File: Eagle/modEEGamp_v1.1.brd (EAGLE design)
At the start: 100 x 80 mm, 115 parts, among them IC201 TLC277P, IC202 INA114P, IC203 INA114P, IC204 TLC277P, IC205 TLC277P, IC206 TLC277P, J201 PINHD-2X17, P201 20k, P202 20k, P203 20k, Q201 BC557, Q202 BC557, Q203 BC557, Q204 BC557, Q205 BC547, Q206 BC547, Q207 BC547, Q208 BC547

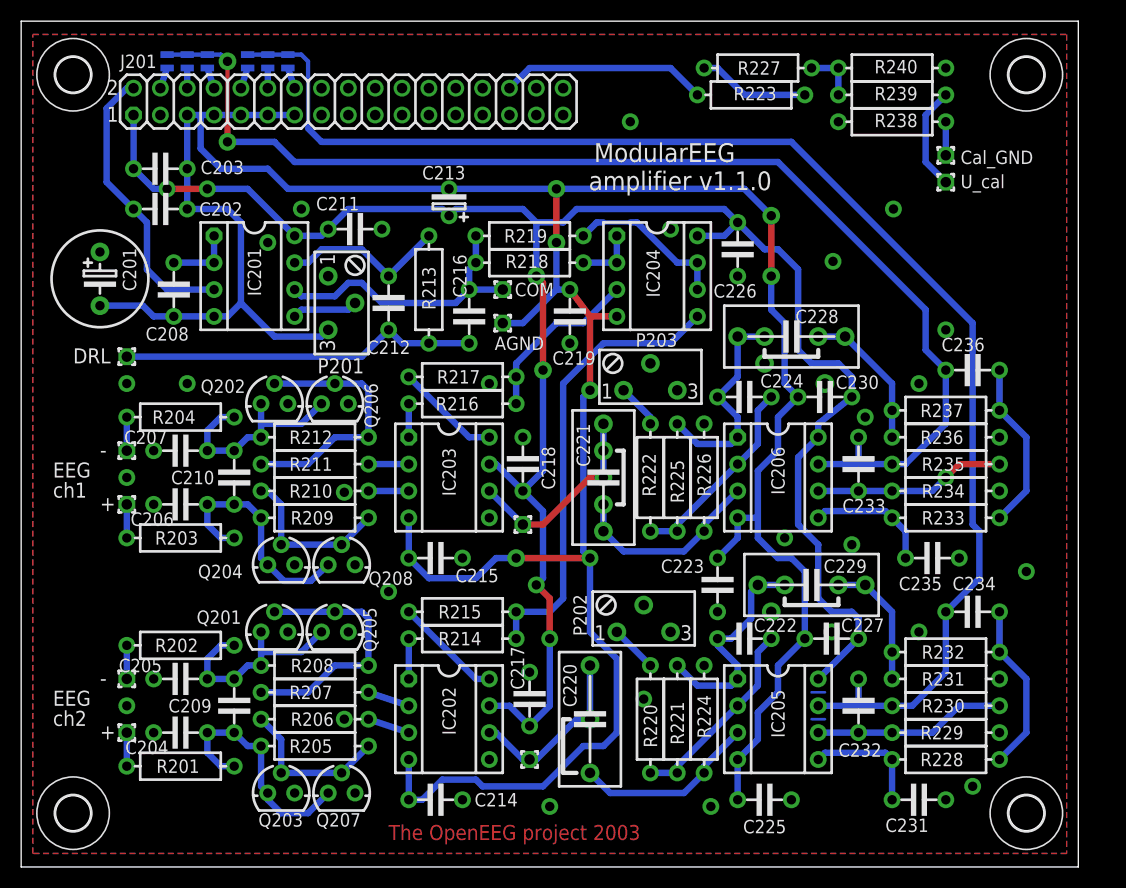
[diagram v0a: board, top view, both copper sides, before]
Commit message: New version!
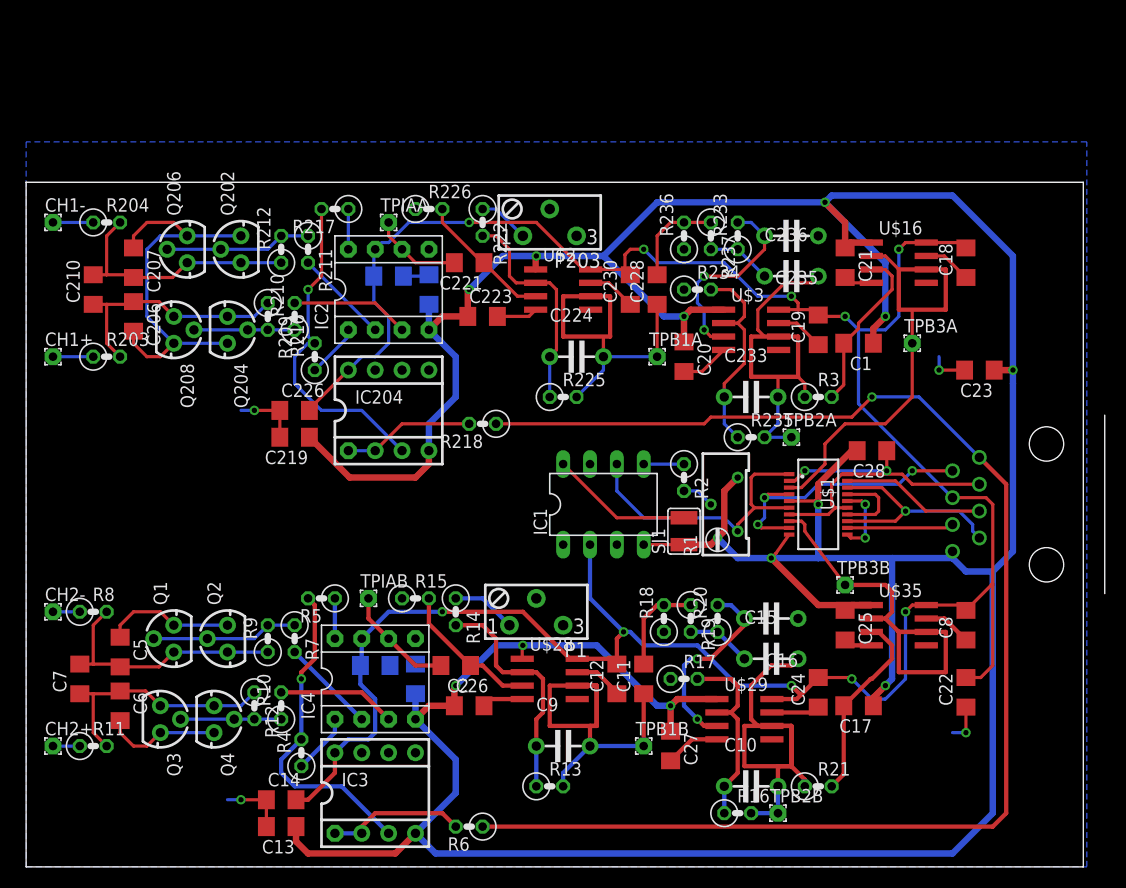
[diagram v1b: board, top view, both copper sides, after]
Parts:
- removed C201: 47µF tan 1ohm, MODEEG:ES-5
- removed C202, C203: 10nF, MODEEG:C-5
- removed C204, C205: 100pF, MODEEG:C-5
- removed C208, C211, C214, C217, C225, C227: 100nF, MODEEG:C-5
- removed C209: 10pF, MODEEG:C-5
- removed C212, C216, C222, C232: 1nF, MODEEG:C-5
- removed C213: 47µF, MODEEG:EL25B
- removed C220, C229: 1µF, MODEEG:C-10
- removed C231: 220nF 5%, MODEEG:C-5
- removed C234: 33nF 5%, MODEEG:C-5
- removed IC201, IC205, IC206: TLC277P, MODEEG:DIL-08
- removed IC202, IC203: INA114P, MODEEG:DIL-08
- removed J201: PINHD-2X17, MODEEG:2X17
- removed P201, P202: 20k, MODEEG:S64Y
- removed PAD201, PAD202, R_LEG: (no value), MODEEG:WIREPAD1
- removed PAD203: U_cal, MODEEG:WIREPAD1
- removed PAD204: Cal_GND, MODEEG:WIREPAD1
- removed PAD205: COM, MODEEG:WIREPAD1
- removed PAD206: AGND, MODEEG:WIREPAD1
- removed Q201, Q203: BC557, MODEEG:TO92
- removed Q205, Q207: BC547, MODEEG:TO92
- removed R201, R202, R205, R206, R207, R208, R214, R215: 2k2, MODEEG:R-10
- removed R213: 200k, MODEEG:R-10
- removed R219, R232, R238, R239: 10k, MODEEG:R-10
- removed R220: 1k, MODEEG:R-10
- removed R221, R230: 100k, MODEEG:R-10
- removed R223, R224, R227, R231: 1M, MODEEG:R-10
- removed R228: 15k, MODEEG:R-10
- removed R229: 8.2k, MODEEG:R-10
- removed R240: 100, MODEEG:R-10
- removed SJ201, SJ202, SJ203, SJ204, SJ205, SJ206: SJ, JUMPER:SJ5X5
- removed U$10, U$11, U$12, U$13: (no value), holes:3,3
- added C1, C17: 220nf, resistor:C1206
- added C10, C9: 1nF, DISCRETE:C-5
- added C11, C2: 1µF, resistor:C1206
- added C12, C13, C14, C18, C19, C20, C21, C22, C23, C24, C25, C26, C27, C28, C3, C4, C8: 100nF, resistor:C1206
- added C15: 33nF 5%, DISCRETE:C-5
- added C16: 220nF 5%, DISCRETE:C-5
- added C5, C6: 100pF, resistor:C1206
- added C7: 10pF, resistor:C1206
- added IC1: AD780N, analog-devices:DIL08
- added IC2, IC4: INA217P, burr-brown:DIL08
- added IC3: TLC277P, BURR:DIL-08
- added P1: 20k, TRIMPOT@2:S64Y
- added Q1, Q3: BC547, NPN:TO92
- added Q2, Q4: BC557, pnp:TO92
- added R1: 25k, resistor:RTRIM64Y
- added R10, R11, R12, R4, R5, R7, R8, R9: 2k2, resistor:0207/2V
- added R13, R16: 100k, resistor:0207/2V
- added R14: 1k, resistor:0207/2V
- added R15, R18, R2: 1M, resistor:0207/2V
- added R17: 8.2k, resistor:0207/2V
- added R19, R6: 10k, resistor:0207/2V
- added R20: 15k, resistor:0207/2V
- added R21, R3: 7.5k, resistor:0207/2V
- added SJ1: (no value), jumper:SJW
- added TPB1A, TPB1B, TPB2A, TPB2B, TPB3A, TPB3B, TPIAA, TPIAB: (no value), WIREPAD:1,6/0,8
- added U$1: AD7902, EEG:QSOP20
- added U$16, U$2, U$28, U$29, U$3, U$35: AD8021, EEG:SOIC8
- added X1: RJ45-6L-B, con-tycoelectronics:RJ45-NO-SHIELD
- C206, C207, C210, C215, C218, C219, C223, C226, C230: device MODEEG:C-5 -> resistor:C1206
- C221, C228: device MODEEG:C-10 -> resistor:C1206
- C224, C233, C235, C236: device MODEEG:C-5 -> DISCRETE:C-5
- CH1+, CH1-, CH2+, CH2-: device MODEEG:WIREPAD1 -> WIREPAD:1,6/0,8
- IC204: device MODEEG:DIL-08 -> BURR:DIL-08
- P203: device MODEEG:S64Y -> TRIMPOT@2:S64Y
- Q202, Q204: device MODEEG:TO92 -> pnp:TO92
- Q206, Q208: device MODEEG:TO92 -> NPN:TO92
- R203, R204, R209, R210, R211, R212, R216, R217, R218, R222, R225, R226, R233, R234, R235, R236, R237: device MODEEG:R-10 -> resistor:0207/2V
- moved C226 44.6 mm to (25.4, 43.2), turned to 0 degrees
- moved R226 36.4 mm to (38.1, 62.2), turned to 0 degrees
- moved C223 33.8 mm to (43.2, 52.1), turned to 0 degrees
- moved C235 33.3 mm to (72.4, 59.7)
- moved R233 33.1 mm to (67.3, 59.7), turned to 90 degrees
- moved R236 31.2 mm to (62.2, 59.7), turned to 90 degrees
- moved R234 30.2 mm to (63.5, 54.6), turned to 0 degrees
- moved R222 28.9 mm to (43.2, 61.0)
- moved C219 28.4 mm to (25.4, 40.6), turned to 180 degrees
- moved IC204 28.4 mm to (34.3, 43.2), turned to 0 degrees
- moved R237 27.7 mm to (64.8, 59.7), turned to 270 degrees
- moved Q208 27.3 mm to (14.0, 50.8), turned to 270 degrees
- moved C215 25.4 mm to (38.1, 54.6), flipped to the bottom, turned to 90 degrees
- moved C221 24.0 mm to (41.9, 57.1), turned to 180 degrees
- moved Q204 22.8 mm to (19.1, 50.8), turned to 270 degrees
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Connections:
- removed net 2.0V: C202.1, IC201.3, J201.2
- removed net PWM: J201.30, R223.2
- removed net R_LEG: C212.1, C216.1, R213.1, R_LEG.1
- removed net VGND: C201.1, C204.2, C205.1, C206.2, C207.1, C208.1, C211.1, C214.2, C215.2, C217.2, C218.2, C219.2, C223.2, C225.2, C226.1, C231.1, C235.1, IC201.1, IC201.2, IC202.5, IC203.5, J201.3, P201.1, P202.2, P202.3, P203.2, P203.3, Q201.1, Q202.1, Q203.1, Q204.1, Q205.1, Q206.1, Q207.1, Q208.1, R224.1, R226.1, R229.1, R231.1, R234.1, R236.1, R238.2, R240.1
- new net N$55: C18.1, U$16.7
- new net N$56: C19.1, U$3.7
- new net N$58: C20.2, U$3.4
- new net N$59: C21.2, U$16.4
- new net N$60: C8.1, U$35.7
- new net N$61: C12.1, U$28.7
- new net N$62: C24.1, U$29.7
- new net N$63: C25.2, U$35.4
- new net N$64: C26.2, U$28.4
- new net N$65: C27.2, U$29.4
- new net N$66: R218.1, R6.1, X1.1
- new net N$67: U$1.12, X1.6
- new net N$68: U$1.19, X1.5
- new net VDD: C28.1, U$1.15, U$1.2, U$1.20, U$1.7, X1.3
- new net VREF: C13.2, C14.1, C16.1, C206.2, C207.1, C215.2, C218.2, C219.2, C22.1, C226.1, C23.2, C235.1, C3.2, C4.2, C5.1, C6.2, IC2.5, IC4.5, P1.2, P1.3, P203.2, P203.3, Q1.1, Q2.1, Q202.1, Q204.1, Q206.1, Q208.1, Q3.1, Q4.1, R15.1, R17.1, R18.1, R226.1, R234.1, R236.1, U$1.4, U$1.9, X1.2
- net +5V/2: now also C12.2, C14.2, C18.2, C19.2, C22.2, C24.2, C3.1, C8.2, IC1.2, IC2.7, IC3.8, IC4.7, U$16.8, U$2.8, U$28.8, U$29.8, U$3.8, U$35.8, X1.4; no longer C203.1, C211.2, C213.1, C217.1, C227.2, IC201.8, IC202.7, IC203.7, IC205.8, IC206.8, J201.1
- net ADIN0: now also TPB3A.1, U$1.3, U$16.2, U$16.6; no longer C233.2, C236.2, IC206.7, R235.2, SJ201.2, SJ202.2, SJ203.2
- net ADIN1: now also TPB3B.1, U$1.8, U$35.2, U$35.6; no longer C232.2, C234.2, IC205.7, R230.2, SJ204.2, SJ205.2, SJ206.2
- net AGND: now also C1.1, C13.1, C17.1, C20.1, C21.1, C23.1, C25.1, C26.1, C27.1, C28.2, C4.1, IC1.4, IC2.4, IC3.4, IC4.4, R1.3, SJ1.1, U$1.10, U$1.5, U$16.1, U$2.1, U$28.1, U$29.1, U$3.1, U$35.1, X1.8; no longer C201.2, C202.2, C203.2, C208.2, C213.2, C214.1, C225.1, C227.1, C230.1, IC201.4, IC202.4, IC203.4, IC205.4, IC206.4, J201.11, J201.13, J201.5, J201.7, J201.9, P201.3, PAD206.1
- net N$1: now also IC1.6, R1.1, U$1.1, U$1.6; no longer IC202.1, R214.1
- net N$10: now also C1.2, R3.2, U$16.3; no longer Q203.2, Q207.2, R205.2, R206.1
- net N$13: now also IC3.3, R4.2, R5.2; no longer C204.1, C209.1, Q203.3, Q207.3, R201.2, R205.1
- net N$14: now also IC2.1; no longer IC203.1
- net N$15: now also C2.2, IC4.6, TPIAB.1; no longer CH2-.1, R202.1
- net N$16: now also IC4.2, R7.2; no longer CH2+.1, R201.1
- net N$17: now also IC4.3, R10.2; no longer C220.1, IC205.3, R224.2
- net N$18: now also Q1.2, Q2.2, R7.1, R9.2; no longer C222.1, IC205.2, R220.2, R221.1
- net N$19: now also C5.2, C7.2, Q1.3, Q2.3, R8.2, R9.1; no longer P202.1, R220.1
- net N$2: now also R1.2, R2.2; no longer IC202.8, R215.1
- net N$20: now also IC2.8; no longer IC203.8
- net N$21: now also IC2.2; no longer IC203.2
- net N$22: now also Q3.2, Q4.2, R10.1, R12.2; no longer C222.2, C229.1, IC205.1, R221.2
- net N$23: now also C6.1, C7.1, Q3.3, Q4.3, R11.2, R12.1; no longer C229.2, R231.2, R232.1
- net N$24: now also CH2-.1, R8.1; no longer C232.1, IC205.6, R229.2, R230.1
- net N$25: now also IC2.6, TPIAA.1; no longer IC203.6, PAD202.1
- net N$26: now also CH2+.1, R11.1; no longer J201.4, SJ201.1
- net N$27: now also IC2.3; no longer IC203.3
- net N$28: now also U$2.3; no longer IC206.3
- net N$3: now also IC1.5, R2.1; no longer IC204.5, R214.2, R215.2
- net N$30: now also C2.1, R15.2, U$28.3; no longer PAD204.1, R238.1
- net N$31: now also C9.1, R13.1, R14.2, U$28.2; no longer J201.6, SJ202.1
- net N$33: now also P1.1, R14.1; no longer C212.2, IC201.7, R213.2
- net N$34: now also C11.1, C9.2, R13.2, TPB1B.1, U$28.6; no longer R227.1, R239.2, R240.2
- net N$35: now also IC3.1, IC3.2, R6.2; no longer J201.8, SJ203.1
- net N$36: now also C15.1, R19.2, R20.1; no longer J201.10, SJ204.1
- net N$37: now also C16.2, R20.2, U$29.3; no longer J201.12, SJ205.1
- net N$38: now also U$2.2; no longer IC206.2
- net N$4: now also U$1.14, U$1.17; no longer C220.2, IC202.6, PAD201.1
- net N$41: now also C11.2, R18.2, R19.1; no longer C216.2, IC201.6, PAD205.1, R218.1, R219.1
- net N$42: now also TPB1A.1, U$2.6; no longer IC206.1
- net N$44: now also C10.1, R16.1, R17.2, U$29.2; no longer J201.14, SJ206.1
- net N$45: now also IC4.1, R4.1; no longer IC204.6, IC204.7, R219.2
- net N$46: now also IC4.8, R5.1; no longer R223.1, R227.2
- net N$47: now also C10.2, C15.2, R16.2, R21.1, TPB2B.1, U$29.6; no longer IC201.5, P201.2
- net N$48: now also C17.2, R21.2, U$35.3; no longer PAD203.1, R239.1
- net N$49: now also U$3.2; no longer IC206.6
- net N$5: now also C233.2, C236.2, R235.2, R3.1, TPB2A.1, U$3.6; no longer IC202.2, R207.2
- net N$53: now also C230.1, U$2.7; no longer C234.1, R228.1, R232.2
- net N$54: now also C223.2, U$2.4; no longer C231.2, IC205.5, R228.2
- net N$57: now also U$3.3; no longer IC206.5
- net N$7: now also U$1.13, U$1.18, X1.7; no longer IC202.3, R206.2
- net N$8: now also U$1.11, U$1.16; no longer Q201.2, Q205.2, R207.1, R208.2
- net N$9: now also IC1.8, SJ1.2; no longer C205.2, C209.2, Q201.3, Q205.3, R202.2, R208.1
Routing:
- net N$66: track 0.00 -> 133.9 mm, vias 0 -> 1
- net ADIN1: track 133.3 -> 21.8 mm
- net VREF: track 0.00 -> 110.6 mm, vias 0 -> 7
- net AGND: track 298.8 -> 406.0 mm, vias 7 -> 13
- net ADIN0: track 114.0 -> 35.4 mm, vias 2 -> 0
- net +5V/2: track 189.5 -> 246.7 mm, vias 6 -> 10
- net N$3: track 43.2 -> 3.81 mm
- net VDD: track 0.00 -> 34.8 mm, vias 0 -> 2
- net R_LEG: track 34.0 -> 0.00 mm
- net 2.0V: track 27.3 -> 0.00 mm
- net N$5: track 4.02 -> 29.7 mm
- net N$1: track 3.81 -> 28.4 mm
- net N$47: track 6.24 -> 27.2 mm
- net N$31: track 1.91 -> 22.3 mm
- net PWM: track 19.6 -> 0.00 mm
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- added copper zone on layer 16, net VREF
- removed copper zone on layer 1, net VGND
- removed copper zone on layer 16, net VGND
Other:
- board size 100 x 80 mm -> 100 x 64.8 mm
- board text removed: "+"
- board text removed: "-"
- board text removed: "1"
- board text removed: "2"
- board text removed: "DRL"
- board text removed: "EEG"
- board text removed: "ModularEEG"
- board text removed: "The OpenEEG project 2003"
- board text removed: "amplifier v1.1.0"
- board text removed: "ch1"
- board text removed: "ch2"
